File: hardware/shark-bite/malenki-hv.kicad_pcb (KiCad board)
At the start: 2 copper layers, 56.9 x 61.3 mm, 108 parts, among them J1 Conn_01x02_Male-Connector, J2 Conn_01x08_Male, J3 Conn_01x02, J4 Conn_01x02_Male-Connector, J5 Conn_01x02_Male-Connector, J6 Conn_01x03_Pin, U1 GM7333, U10 IRFH7440TRPBF, U11 IRFH7440TRPBF, U12 IRFH7440TRPBF, U13 DRV8231DSGR, U14 DRV8231DSGR, U2 ATTiny1616-MNR, U3 A7105, U4 GD32E230G6U6TR, U5 FD6288Q, U6 AOZ1282CI, U7 IRFH7440TRPBF, U8 IRFH7440TRPBF, U9 IRFH7440TRPBF, Y1 16mhz Seiko Epson Q24FA20H005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

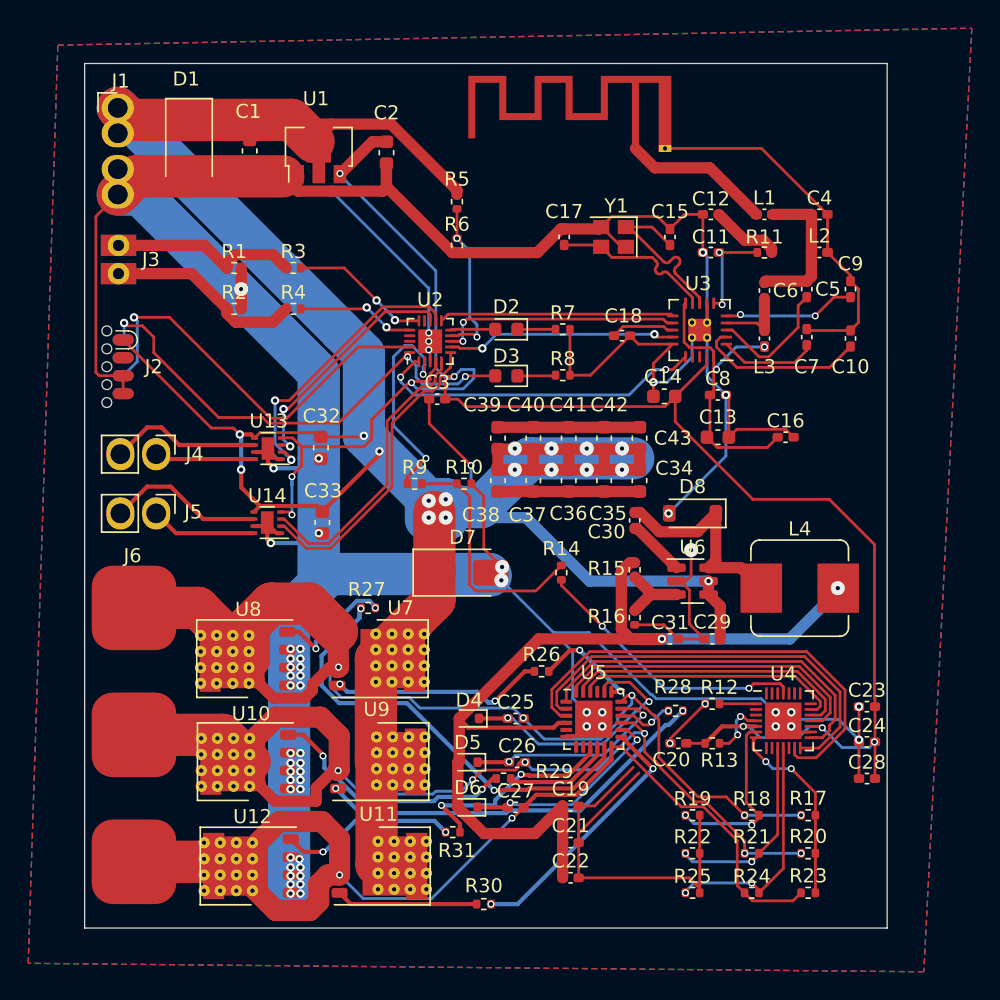
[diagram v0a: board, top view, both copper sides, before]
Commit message: Minor Changes???
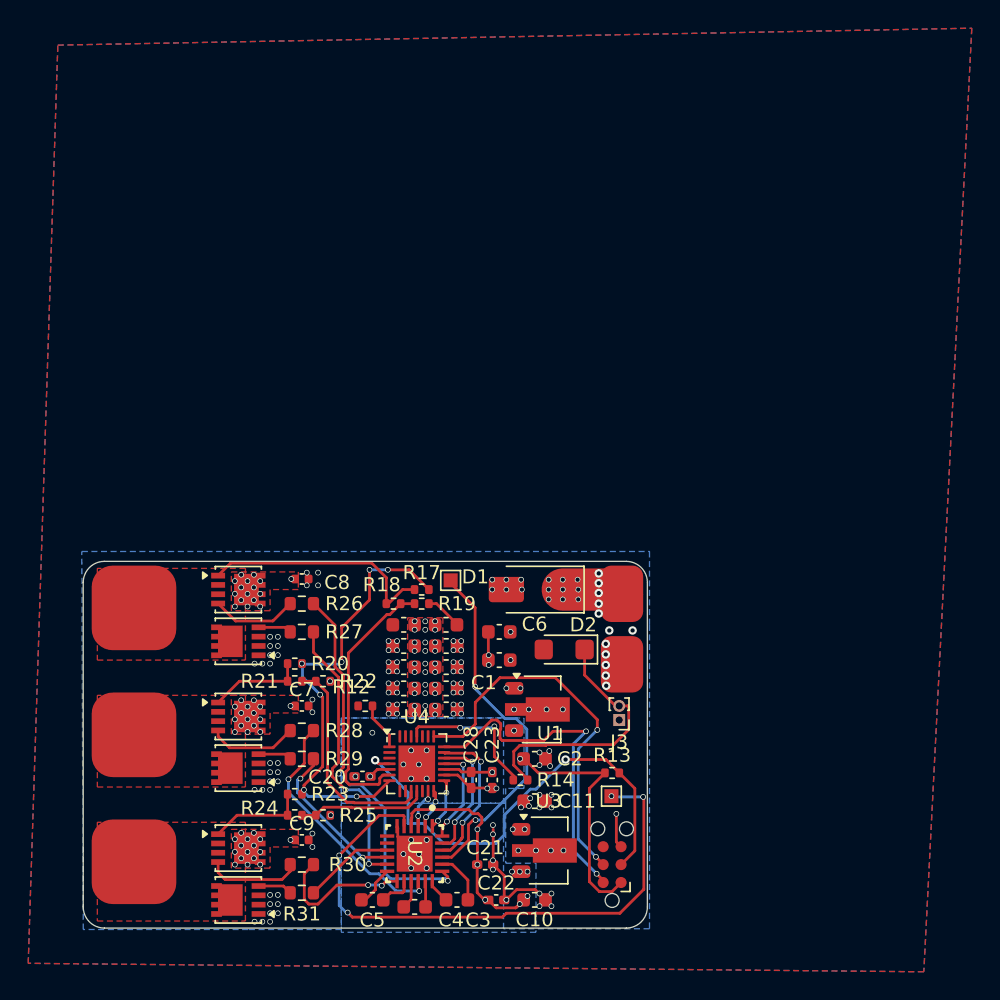
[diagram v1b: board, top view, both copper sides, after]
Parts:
- removed AE1: ~, malenki-nano:malenki_antenna
- removed C12: 10nF, Capacitor_SMD:C_0402_1005Metric_Pad0.74x0.62mm_HandSolder
- removed C13, C14: 2.2uF, Capacitor_SMD:C_0603_1608Metric
- removed C15, C17: 10pF, Capacitor_SMD:C_0402_1005Metric_Pad0.74x0.62mm_HandSolder
- removed C16, C18, C19, C30: 100nF, Capacitor_SMD:C_0402_1005Metric_Pad0.74x0.62mm_HandSolder
- removed C24, C25, C26, C27: 1uF, Capacitor_SMD:C_0402_1005Metric_Pad0.74x0.62mm_HandSolder
- removed C29, C31: 10uF, Capacitor_SMD:C_0402_1005Metric_Pad0.74x0.62mm_HandSolder
- removed C32, C33: 10uF 25V, Capacitor_SMD:C_0603_1608Metric
- removed D3: LED Red, LED_SMD:LED_0603_1608Metric
- removed D4, D5, D6: 1N4148WT, Diode_SMD:D_SOD-523
- removed D7: SMAJ18A, Diode_SMD:D_SMA
- removed D8: B5817W, Diode_SMD:D_SOD-123
- removed J4, J5: Conn_01x02_Male-Connector, malenki-nano:PinHeader_1x02_P2.54mm_BIG1
- removed L1: 2.7nH, Inductor_SMD:L_0402_1005Metric_Pad0.77x0.64mm_HandSolder
- removed L2, L3: 4.7nH, Inductor_SMD:L_0402_1005Metric_Pad0.77x0.64mm_HandSolder
- removed L4: 22uH, Inductor_SMD:L_Bourns_SRP7028A_7.3x6.6mm
- removed R1, R10, R2, R6: 10k, Resistor_SMD:R_0402_1005Metric
- removed R11: 200R, Resistor_SMD:R_0402_1005Metric
- removed R15: 49.9K, Resistor_SMD:R_0402_1005Metric
- removed R16: 4.32K, Resistor_SMD:R_0402_1005Metric
- removed R3, R4, R7, R9: 470R, Resistor_SMD:R_0402_1005Metric
- removed R5: 100k, Resistor_SMD:R_0402_1005Metric
- removed R8: 1k, Resistor_SMD:R_0402_1005Metric
- removed U13, U14: DRV8231DSGR, Package_SON:WSON-8-1EP_2x2mm_P0.5mm_EP0.9x1.6mm
- removed U5: FD6288Q, Package_DFN_QFN:QFN-24-1EP_4x4mm_P0.5mm_EP2.65x2.65mm
- removed U6: AOZ1282CI, Package_TO_SOT_SMD:SOT-23-6
- removed Y1: 16mhz Seiko Epson Q24FA20H0051200, Crystal:Crystal_SMD_2520-4Pin_2.5x2.0mm
- added TP1: TestPoint, TestPoint:TestPoint_Pad_1.0x1.0mm, F.Cu at (125.5, 80.7)
- added TP2: TestPoint, TestPoint:TestPoint_Pad_1.0x1.0mm, F.Cu at (114.0, 65.3)
- C1, C2: value 10uF 25V -> 10uF
- C10, C3: value 100nF -> 1uF; footprint Capacitor_SMD:C_0402_1005Metric_Pad0.74x0.62mm_HandSolder -> Capacitor_SMD:C_0603_1608Metric
- C11: value 560pF -> 1uF; footprint Capacitor_SMD:C_0402_1005Metric_Pad0.74x0.62mm_HandSolder -> Capacitor_SMD:C_0603_1608Metric
- C22: value 4.7uF -> 10uF
- C23: value 100nF -> 10nF
- C28: value 4.7uF -> 1uF
- C4: value 1pF -> 1uF; footprint Capacitor_SMD:C_0402_1005Metric_Pad0.74x0.62mm_HandSolder -> Capacitor_SMD:C_0603_1608Metric
- C5: value 22pF -> 1uF; footprint Capacitor_SMD:C_0402_1005Metric_Pad0.74x0.62mm_HandSolder -> Capacitor_SMD:C_0603_1608Metric
- C6: value 10pF -> 330uF; footprint Capacitor_SMD:C_0402_1005Metric_Pad0.74x0.62mm_HandSolder -> Capacitor_SMD:C_0603_1608Metric
- C7, C8, C9: value 100nF -> 1uF; footprint Capacitor_SMD:C_0402_1005Metric_Pad0.74x0.62mm_HandSolder -> Capacitor_SMD:C_0402_1005Metric
- D2: value LED Blue -> SMF5V0A; footprint LED_SMD:LED_0603_1608Metric -> Diode_SMD:D_SMF
- J1: footprint malenki-nano:malenkipower -> Sharkbite:Power Input
- J2: value Conn_01x08_Male -> Conn_ARM_SWD_TagConnect_TC2030-NL; footprint malenki-nano:SOIC_clipProgSmall -> Connector:Tag-Connect_TC2030-IDC-NL_2x03_P1.27mm_Vertical
- J3: value Conn_01x02 -> PWM Pads; footprint malenki-nano:wirepad_2 -> Connector_PinHeader_1.00mm:PinHeader_1x02_P1.00mm_Vertical
- J6: value Conn_01x03_Pin -> Motor Pads
- R14: value 1K -> 100
- R26, R27, R28, R29, R30, R31: value 20 -> 2.2; footprint Resistor_SMD:R_0402_1005Metric -> Resistor_SMD:R_0603_1608Metric
- U10, U11, U12, U7, U8, U9: value IRFH7440TRPBF -> SISS54; footprint Sharkbite:PQFN FET -> Sharkbite:1212-8S
- U2: value ATTiny1616-MNR -> DRV8300DRGER; footprint Package_DFN_QFN:VQFN-20-1EP_3x3mm_P0.4mm_EP1.7x1.7mm -> Sharkbite:RGE0024B-IPC_A
- U3: value A7105 -> ~; footprint malenki-nano:a7105-QFN-20 -> Package_TO_SOT_SMD:SOT-89-3
- moved C4 56.9 mm to (111.5, 88.5), turned to 180 degrees
- moved C9 55.1 mm to (103.5, 83.8), turned to 0 degrees
- moved C5 53.1 mm to (108.5, 88.0), turned to 180 degrees
- moved J2 49.0 mm to (125.5, 85.5)
- moved J1 48.4 mm to (126.2, 66.3)
- moved J3 48.2 mm to (126.0, 75.2), turned to 180 degrees
- moved C10 45.7 mm to (120.0, 88.0), turned to 0 degrees
- moved C7 44.3 mm to (103.5, 74.2), turned to 0 degrees
- moved C2 44.2 mm to (120.0, 78.0), turned to 0 degrees
- moved U1 42.9 mm to (120.5, 74.5), turned to 0 degrees
- moved C11 40.9 mm to (120.0, 81.0)
- moved C1 40.2 mm to (117.5, 71.0), turned to 180 degrees
- moved D1 39.7 mm to (120.0, 66.0), turned to 180 degrees
- moved R20 38.8 mm to (103.0, 71.2)
- moved U3 38.4 mm to (121.0, 84.5), turned to 0 degrees
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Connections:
- net BEMF_A renamed /motor_driver_1_weapon/BEMF_A
- net BEMF_B renamed /motor_driver_1_weapon/BEMF_B
- net BEMF_C renamed /motor_driver_1_weapon/BEMF_C
- net BEMF_COMMON renamed /motor_driver_1_weapon/BEMF_COM
- C1 pad 1: VBAT -> VBUS
- C10 pad 1: Net-(U3-BPBG) -> +10V
- C11 pad 1: GND -> VBUS
- C11 pad 2: Net-(U3-VT) -> GND
- C2 pad 1: VLOGIC -> +3V3
- C20 pad 1: VLOGIC -> +3V3
- C23 pad 2: VLOGIC -> +3V3
- C28 pad 2: VLOGIC -> +3V3
- C3 pad 1: VLOGIC -> Net-(U2-BSTA)
- C3 pad 2: GND -> Net-(U2-SHA)
- C34 pad 1: VBAT -> VBUS
- C35 pad 1: VBAT -> VBUS
- C36 pad 1: VBAT -> VBUS
- C37 pad 1: VBAT -> VBUS
- C38 pad 1: VBAT -> VBUS
- C39 pad 1: VBAT -> VBUS
- C4 pad 1: /radio/IMPMATCH -> Net-(U2-BSTB)
- C4 pad 2: GND -> Net-(U2-SHB)
- C40 pad 1: VBAT -> VBUS
- C41 pad 1: VBAT -> VBUS
- C42 pad 1: VBAT -> VBUS
- C43 pad 1: VBAT -> VBUS
- C5 pad 1: /radio/IMPMATCH -> Net-(U2-BSTC)
- C5 pad 2: /radio/RFI -> Net-(U2-SHC)
- C6 pad 1: /radio/IMPMATCH -> VBUS
- C6 pad 2: /radio/RFO -> GND
- C7 pad 1: Net-(U3-RSSI) -> VBUS
- C8 pad 1: /radio/REGOA -> VBUS
- C9 pad 1: /radio/VDA2 -> VBUS
- D1 pad 1: VBAT -> VBUS
- D2 pad 1: Net-(D2-K) -> /motor_driver_1_weapon/PWM
- D2 pad 2: BLINKY -> GND
- J1 pad 1: VBAT -> VBUS
- J2 pad 1: VBAT -> +3V3
- J2 pad 2: unconnected-(J2-Pin_2-Pad2) -> /motor_driver_1_weapon/SWDIO
- J2 pad 3: GND -> /motor_driver_1_weapon/RST
- J2 pad 4: GND -> /motor_driver_1_weapon/SWDCLK
- J2 pad 5: unconnected-(J2-Pin_5-Pad5) -> GND
- J2 pad 6: UPDI -> unconnected-(J2-SWO-Pad6)
- J3 pad 1: WEAPON3 -> GND
- J3 pad 2: WEAPON2 -> /motor_driver_1_weapon/PWM
- J6 pad 1: OUT_C -> /motor_driver_1_weapon/OUT_C
- J6 pad 2: OUT_B -> /motor_driver_1_weapon/OUT_B
- J6 pad 3: OUT_A -> /motor_driver_1_weapon/OUT_A
- R13 pad 1: VLOGIC -> +3V3
- R13 pad 2: Net-(U4-NRST) -> /motor_driver_1_weapon/RST
- R14 pad 2: MOTOR1 -> /motor_driver_1_weapon/PWM
- R17 pad 2: OUT_A -> /motor_driver_1_weapon/OUT_A
- R18 pad 1: OUT_A -> /motor_driver_1_weapon/OUT_A
- R20 pad 2: OUT_B -> /motor_driver_1_weapon/OUT_B
- R21 pad 1: OUT_B -> /motor_driver_1_weapon/OUT_B
- R23 pad 2: OUT_C -> /motor_driver_1_weapon/OUT_C
- R24 pad 1: OUT_C -> /motor_driver_1_weapon/OUT_C
- R26 pad 1: GATE_HIGH_A -> /motor_driver_1_weapon/GHA
- R27 pad 1: GATE_LOW_A -> /motor_driver_1_weapon/GLA
- R28 pad 2: GATE_HIGH_B -> /motor_driver_1_weapon/GHB
- R29 pad 1: GATE_LOW_B -> /motor_driver_1_weapon/GLB
- R30 pad 2: GATE_HIGH_C -> /motor_driver_1_weapon/GHC
- R31 pad 2: GATE_LOW_C -> /motor_driver_1_weapon/GLC
- U1 pad 2: VBAT -> VBUS
- U1 pad 3: VLOGIC -> +3V3
- U2 pad 1: GIO1 -> /motor_driver_1_weapon/ALOW
- U2 pad 10: BLINKY -> /motor_driver_1_weapon/GLB
- U2 pad 11: SPI_SCS -> /motor_driver_1_weapon/GLA
- U2 pad 12: MOTOR2F -> Net-(U2-SHC)
- U2 pad 13: MOTOR2R -> /motor_driver_1_weapon/GHC
- U2 pad 14: unconnected-(U2-PB0-Pad14) -> Net-(U2-BSTC)
- U2 pad 15: /W2 -> Net-(U2-SHB)
- U2 pad 16: /W3 -> /motor_driver_1_weapon/GHB
- U2 pad 17: unconnected-(U2-PC2-Pad17) -> Net-(U2-BSTB)
- U2 pad 18: unconnected-(U2-PC3-Pad18) -> Net-(U2-SHA)
- U2 pad 19: UPDI -> /motor_driver_1_weapon/GHA
- U2 pad 2: Net-(U2-PA3) -> /motor_driver_1_weapon/BLOW
- U2 pad 20: TXDEBUG -> Net-(U2-BSTA)
- U2 pad 21: GND -> Net-(U2-DT)
- U2 pad 3: GND -> /motor_driver_1_weapon/CLOW
- U2 pad 4: VLOGIC -> +10V
- U2 pad 5: MOTOR3R -> Net-(U2-MODE)
- U2 pad 6: MOTOR3F -> GND
- U2 pad 7: SPI_SDIO -> unconnected-(U2-NC-Pad7)
- U2 pad 8: SPI_SCK -> unconnected-(U2-NC-Pad8)
- U2 pad 9: VSENSE -> /motor_driver_1_weapon/GLC
- U3 pad 1: Net-(U3-RSSI) -> GND
- U3 pad 2: Net-(U3-BPBG) -> VBUS
- U3 pad 3: /radio/RFI -> +10V
- U4 pad 13: CLOW -> /motor_driver_1_weapon/CLOW
- U4 pad 14: BLOW -> /motor_driver_1_weapon/BLOW
- U4 pad 15: ALOW -> /motor_driver_1_weapon/ALOW
- U4 pad 17: VLOGIC -> +3V3
- U4 pad 18: CHIGH -> /motor_driver_1_weapon/CHIGH
- U4 pad 19: BHIGH -> /motor_driver_1_weapon/BHIGH
- U4 pad 20: AHIGH -> /motor_driver_1_weapon/AHIGH
- U4 pad 21: SWDIO -> /motor_driver_1_weapon/SWDIO
- U4 pad 22: SWDCLK -> /motor_driver_1_weapon/SWDCLK
- U4 pad 4: Net-(U4-NRST) -> /motor_driver_1_weapon/RST
- U4 pad 5: VLOGIC -> +3V3
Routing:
- net GND: track 386.2 -> 21.7 mm, vias 58 -> 122
- net VBAT: track 206.1 -> 0.00 mm, vias 17 -> 0
- net VLOGIC: track 127.2 -> 0.00 mm, vias 8 -> 0
- net OUT_A: track 74.0 -> 0.00 mm, vias 5 -> 0
- net OUT_C: track 73.8 -> 0.00 mm, vias 2 -> 0
- net OUT_B: track 71.6 -> 0.00 mm, vias 6 -> 0
- net +10V: track 67.8 -> 15.8 mm, vias 2 -> 8
- net Net-(U2-MODE): track 0.00 -> 41.6 mm, vias 0 -> 4
- net TXDEBUG: track 35.2 -> 0.00 mm, vias 3 -> 0
- net CLOW: track 33.3 -> 0.00 mm
- net /motor_driver_1_weapon/RST: track 0.00 -> 33.2 mm, vias 0 -> 2
- net GATE_LOW_A: track 32.2 -> 0.00 mm, vias 2 -> 0
- net BLOW: track 29.8 -> 0.00 mm
- net UPDI: track 29.2 -> 0.00 mm, vias 1 -> 0
- net /motor_driver_1_weapon/GHA: track 0.00 -> 27.5 mm, vias 0 -> 2
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- added copper zone on B.Cu, net +10V
- added copper zone on B.Cu, net +3V3
- added copper zone on F.Cu, net /motor_driver_1_weapon/OUT_A
- added copper zone on F.Cu, net /motor_driver_1_weapon/OUT_B
- added copper zone on F.Cu, net /motor_driver_1_weapon/OUT_C
- added copper zone on In1.Cu, net GND
- added copper zone on In2.Cu, net GND
- added copper zone on B.Cu, net VBUS
- added copper zone on F.Cu, net VBUS
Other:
- board size 56.9 x 61.3 mm -> 40 x 26 mm
- copper layers 2 -> 4
